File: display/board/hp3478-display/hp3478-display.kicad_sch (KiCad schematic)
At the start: 2 parts, among them U1 PIC16F15274-I/MP, U2 DNP

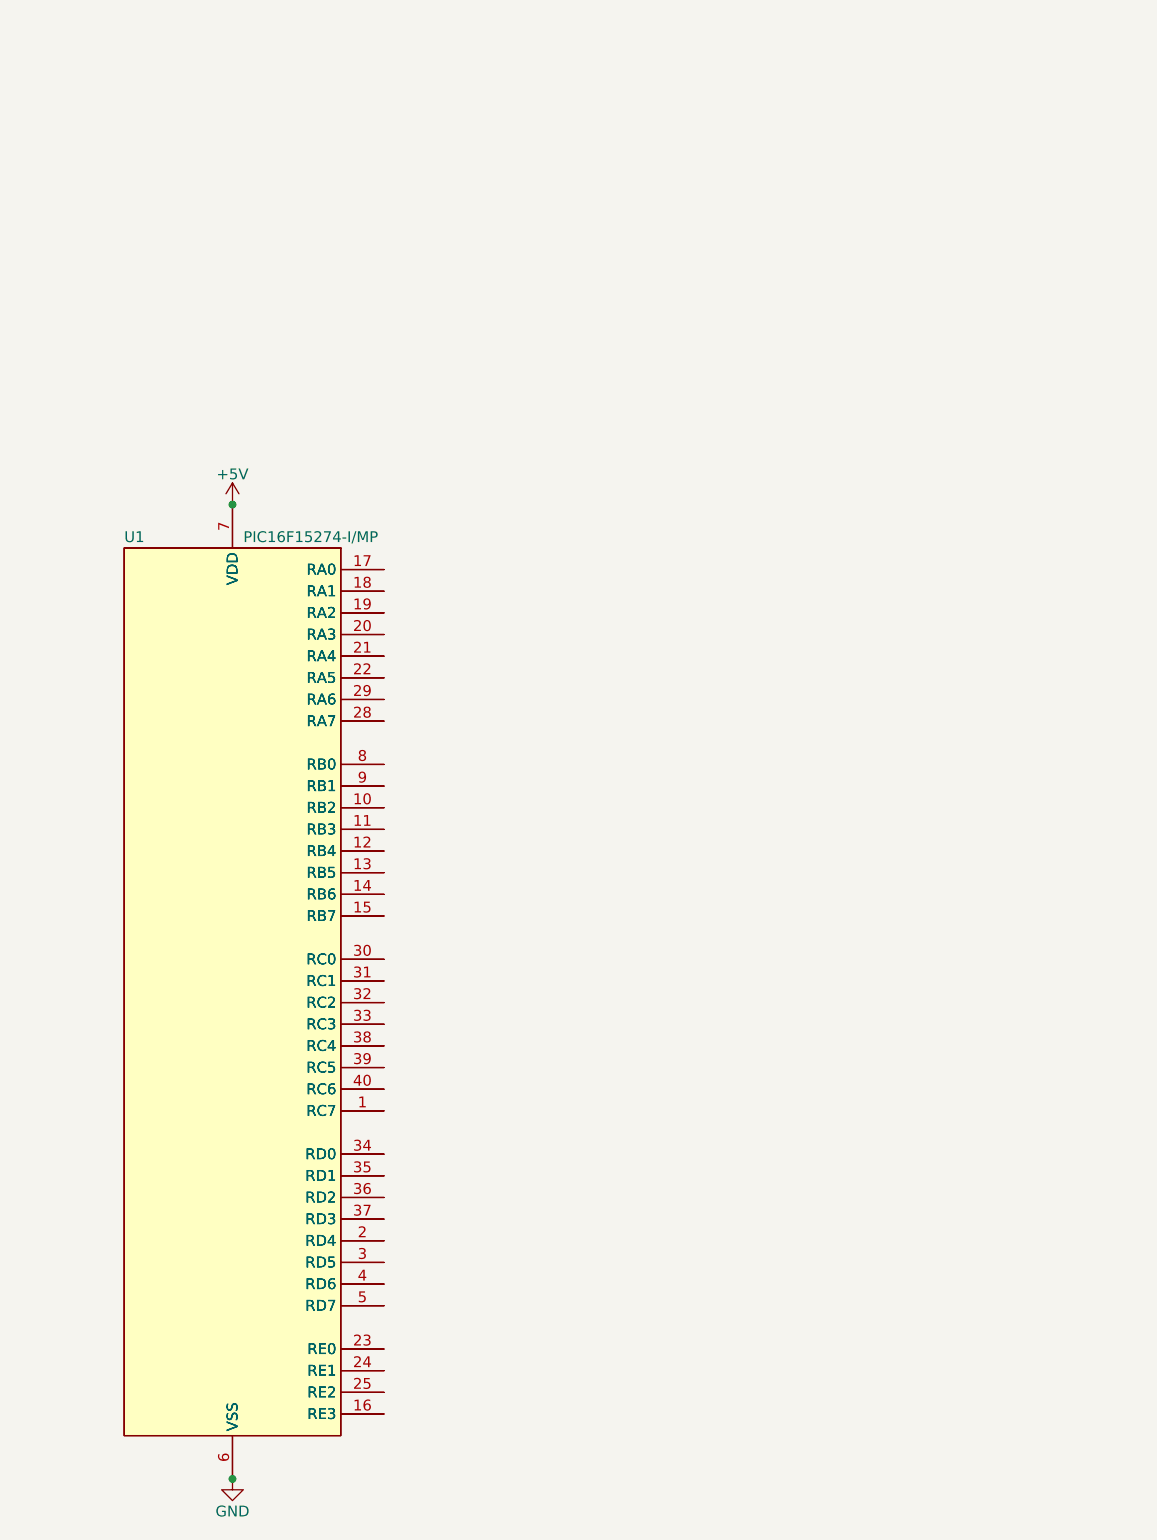
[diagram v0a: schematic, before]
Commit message: Assign all pins.
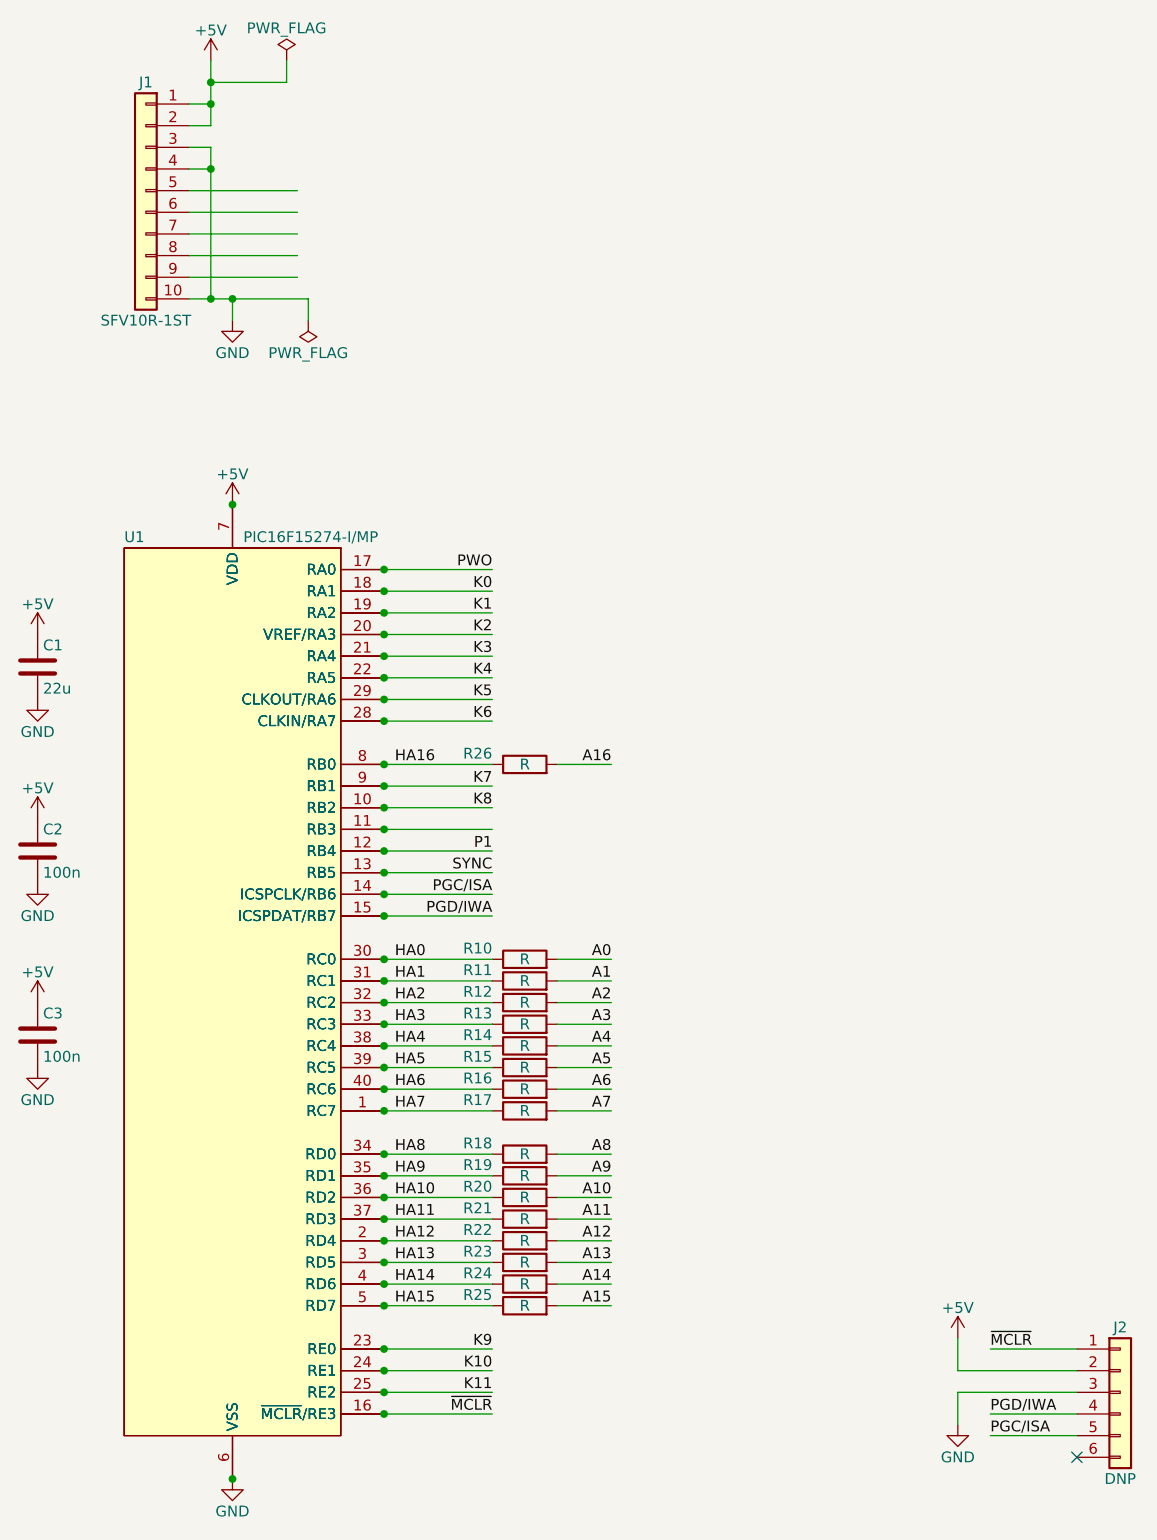
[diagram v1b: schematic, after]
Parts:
- added C1: 22u, Capacitor_SMD:C_1206_3216Metric, symbol Device:C
- added C2, C3: 100n, Capacitor_SMD:C_0603_1608Metric, symbol Device:C
- added J1: SFV10R-1ST, 0Local:Amphenol_SFV10R-1ST, symbol Connector_Generic:Conn_01x10
- added J2: DNP, Connector_PinHeader_2.54mm:PinHeader_1x06_P2.54mm_Vertical, symbol Connector_Generic:Conn_01x06
- added R10, R11, R12, R13, R14, R15, R16, R17, R18, R19, R20, R21, R22, R23, R24, R25, R26: R, Resistor_SMD:R_0603_1608Metric, symbol Device:R
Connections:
- net +5V: now also C1.1, C2.1, C3.1, J1.1 (Pin_1), J1.2 (Pin_2), J2.2 (Pin_2)
- net GND: now also C1.2, C2.2, C3.2, J1.10 (Pin_10), J1.3 (Pin_3), J1.4 (Pin_4), J2.3 (Pin_3)
- net HA7: now reaches U1.1 (RC7), U2.1 (RC7)
- net HA7: now also R17.1
- net K8: now reaches U1.10 (RB2), U2.10 (RB2)
- net P1: now reaches U1.12 (RB4), U2.14 (RB4)
- net SYNC: now reaches U1.13 (RB5), U2.15 (RB5)
- net PGC/ISA: now reaches U1.14 (ICSPCLK/RB6), U2.16 (ICSPCLK/RB6)
- net PGC/ISA: now also J2.5 (Pin_5)
- net PGD/IWA: now reaches U1.15 (ICSPDAT/RB7), U2.17 (ICSPDAT/RB7)
- net PGD/IWA: now also J2.4 (Pin_4)
- net ~{MCLR}: now reaches U1.16 (~{MCLR}/RE3), U2.18 (~{MCLR}/RE3)
- net ~{MCLR}: now also J2.1 (Pin_1)
- net PWO: now reaches U1.17 (RA0), U2.19 (RA0)
- net HA12: now reaches U1.2 (RD4), U2.2 (RD4)
- net HA12: now also R22.1
- net K0: now reaches U1.18 (RA1), U2.20 (RA1)
- net K1: now reaches U1.19 (RA2), U2.21 (RA2)
- net K2: now reaches U1.20 (VREF/RA3), U2.22 (VREF/RA3)
- net K3: now reaches U1.21 (RA4), U2.23 (RA4)
- net K4: now reaches U1.22 (RA5), U2.24 (RA5)
- net K9: now reaches U1.23 (RE0), U2.25 (RE0)
- net K10: now reaches U1.24 (RE1), U2.26 (RE1)
- net K11: now reaches U1.25 (RE2), U2.27 (RE2)
- net HA13: now reaches U1.3 (RD5), U2.3 (RD5)
- net HA13: now also R23.1
- net K6: now reaches U1.28 (CLKIN/RA7), U2.30 (CLKIN/RA7)
- net K5: now reaches U1.29 (CLKOUT/RA6), U2.31 (CLKOUT/RA6)
- net HA0: now reaches U1.30 (RC0), U2.32 (RC0)
- net HA0: now also R10.1
- net HA1: now reaches U1.31 (RC1), U2.35 (RC1)
- net HA1: now also R11.1
- net HA2: now reaches U1.32 (RC2), U2.36 (RC2)
- net HA2: now also R12.1
- net HA3: now reaches U1.33 (RC3), U2.37 (RC3)
- net HA3: now also R13.1
- net HA8: now reaches U1.34 (RD0), U2.38 (RD0)
- net HA8: now also R18.1
- net HA9: now reaches U1.35 (RD1), U2.39 (RD1)
- net HA9: now also R19.1
- net HA14: now reaches U1.4 (RD6), U2.4 (RD6)
- net HA14: now also R24.1
- net HA10: now reaches U1.36 (RD2), U2.40 (RD2)
- net HA10: now also R20.1
- net HA11: now reaches U1.37 (RD3), U2.41 (RD3)
- net HA11: now also R21.1
- net HA4: now reaches U1.38 (RC4), U2.42 (RC4)
- net HA4: now also R14.1
- net HA5: now reaches U1.39 (RC5), U2.43 (RC5)
- net HA5: now also R15.1
- net HA6: now reaches U1.40 (RC6), U2.44 (RC6)
- net HA6: now also R16.1
- net HA15: now reaches U1.5 (RD7), U2.5 (RD7)
- net HA15: now also R25.1
- net HA16: now reaches U1.8 (RB0), U2.8 (RB0)
- net HA16: now also R26.1
- net K7: now reaches U1.9 (RB1), U2.9 (RB1)
- new net A0: R10.2
- new net A1: R11.2
- new net A10: R20.2
- new net A11: R21.2
- new net A12: R22.2
- new net A13: R23.2
- new net A14: R24.2
- new net A15: R25.2
- new net A16: R26.2
- new net A2: R12.2
- new net A3: R13.2
- new net A4: R14.2
- new net A5: R15.2
- new net A6: R16.2
- new net A7: R17.2
- new net A8: R18.2
- new net A9: R19.2
- no-connect marks 0 -> 1
